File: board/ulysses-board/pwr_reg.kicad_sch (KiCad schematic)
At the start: 35 parts, among them J2 8V-30V, Q1 IRF9540N, Q2 2N3906, Q3 IRF9540N, Q4 2N3906, SW1 On/Off, SW2 RESET, U1 LM350, U2 LM350, U3 LM350

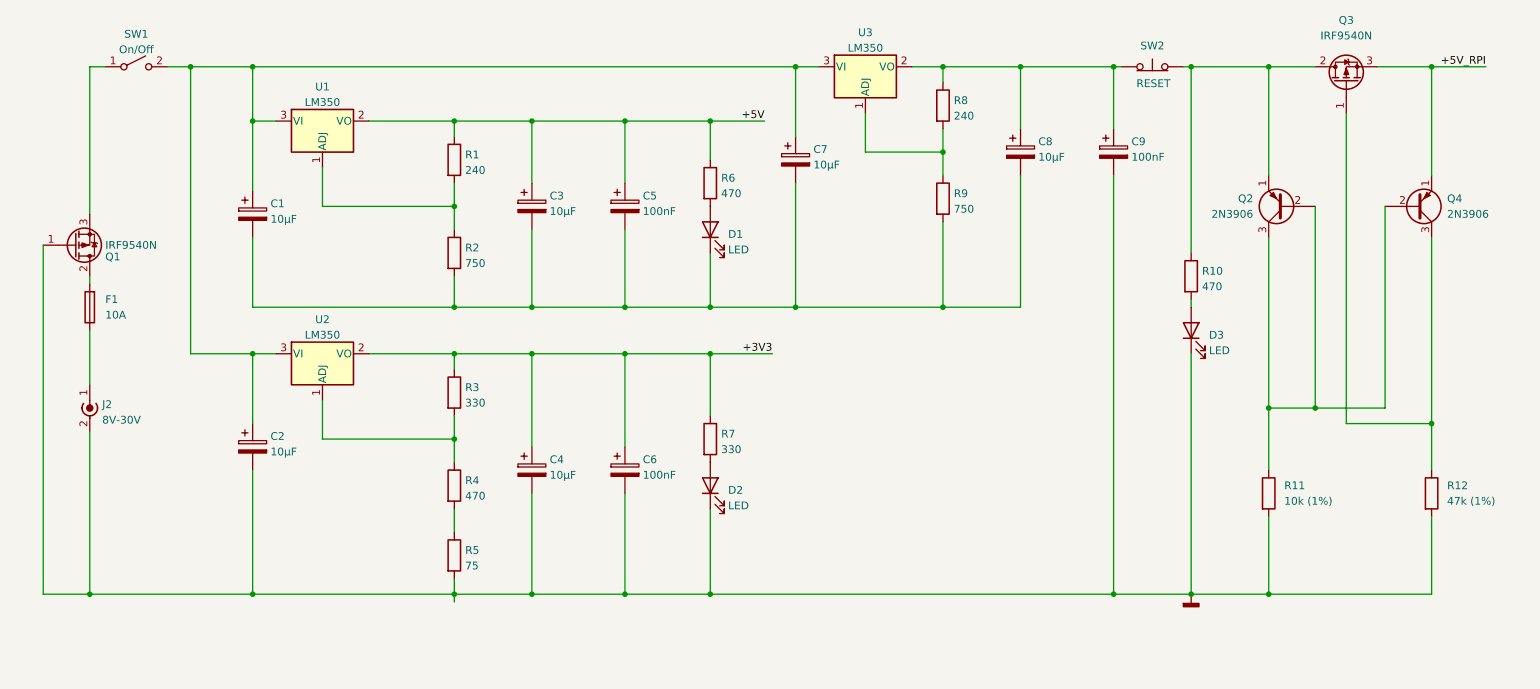
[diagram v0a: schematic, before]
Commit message: Some minor imptovements.
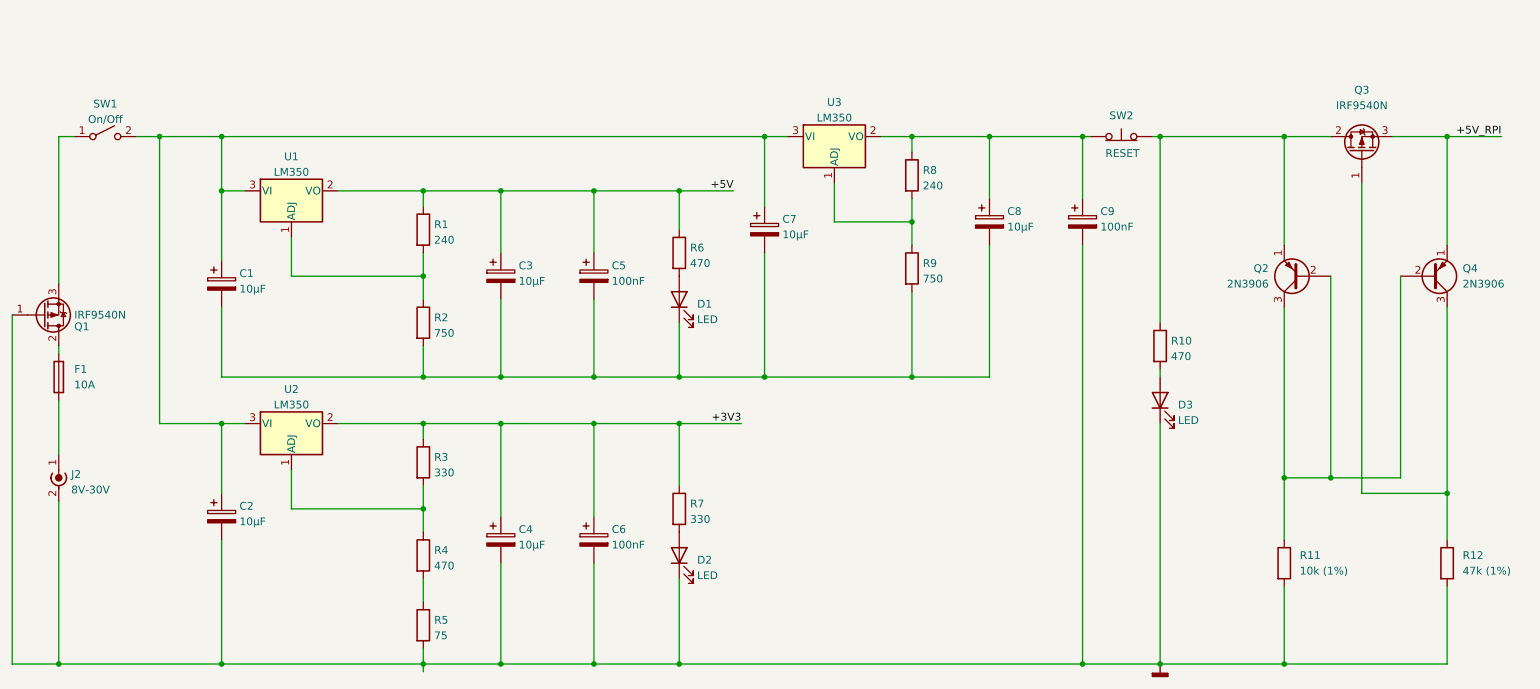
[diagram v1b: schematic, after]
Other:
- moved on the sheet: C1, C2, C3, C4, C5, C6, C7, C8, C9, D1, D2, D3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
